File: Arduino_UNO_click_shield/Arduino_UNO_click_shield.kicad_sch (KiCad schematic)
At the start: 14 parts, among them J1 mikroBUS host connector, J2 mikroBUS host connector, J4 UPDI, U1 ATtiny1616-M

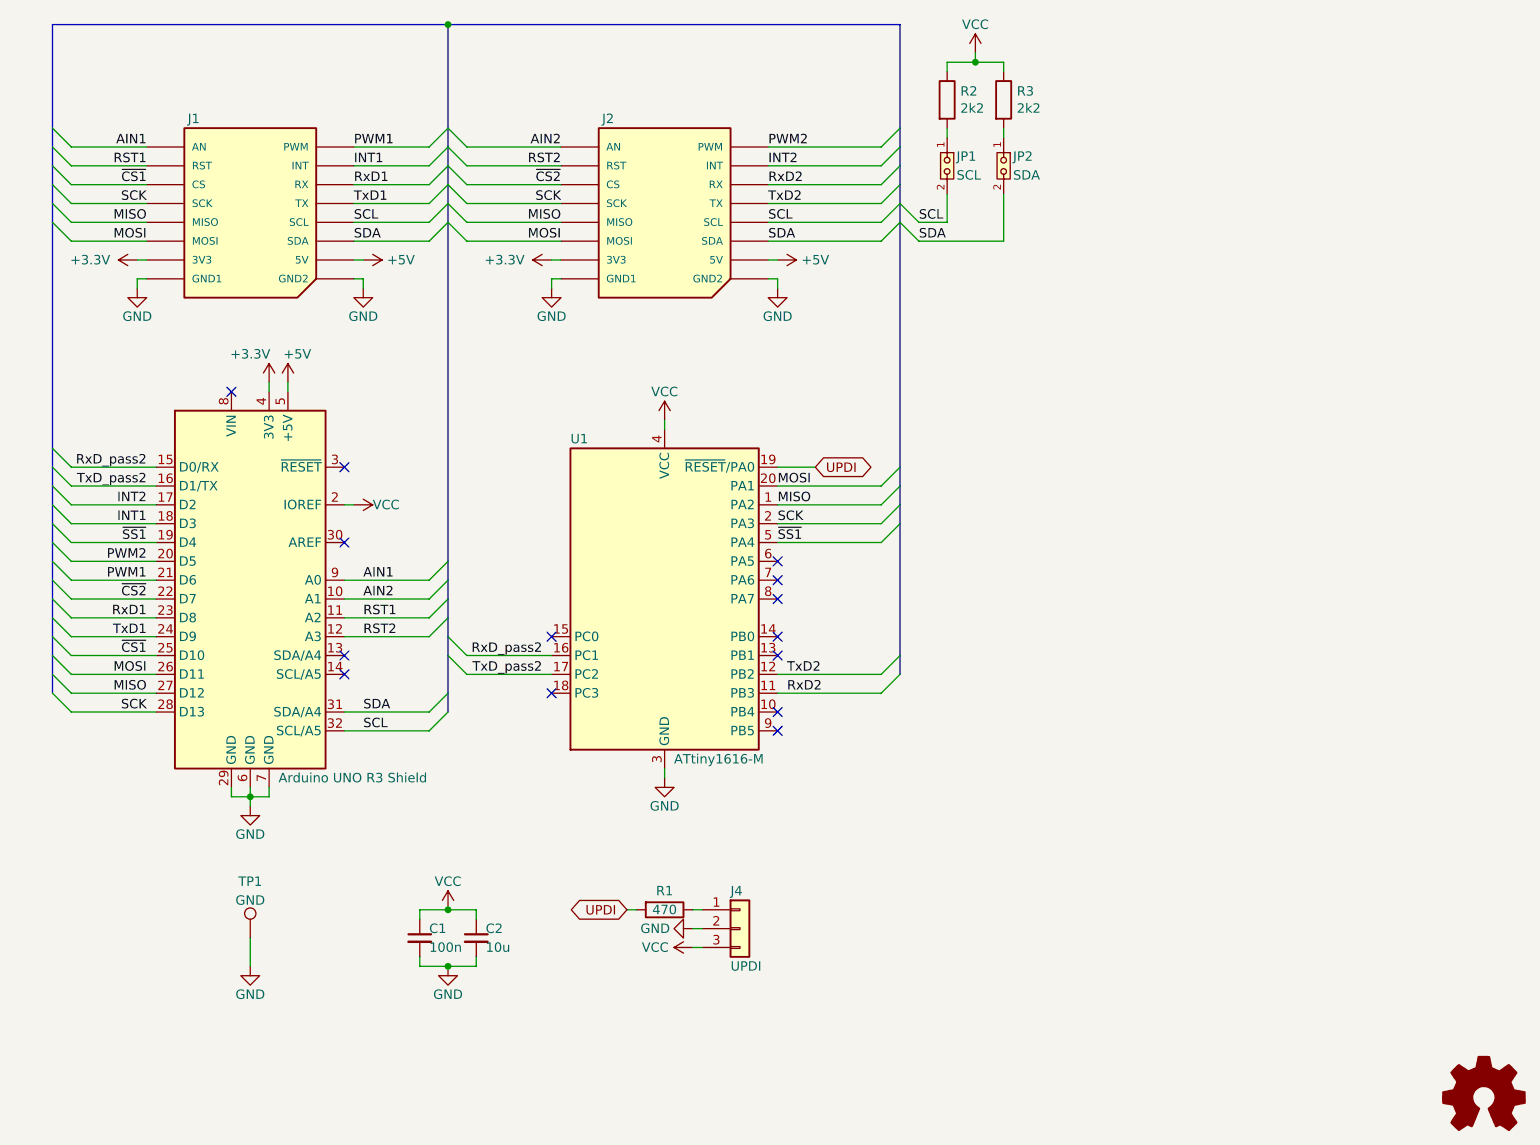
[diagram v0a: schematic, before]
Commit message: Arduino UNO Click shield v1.2
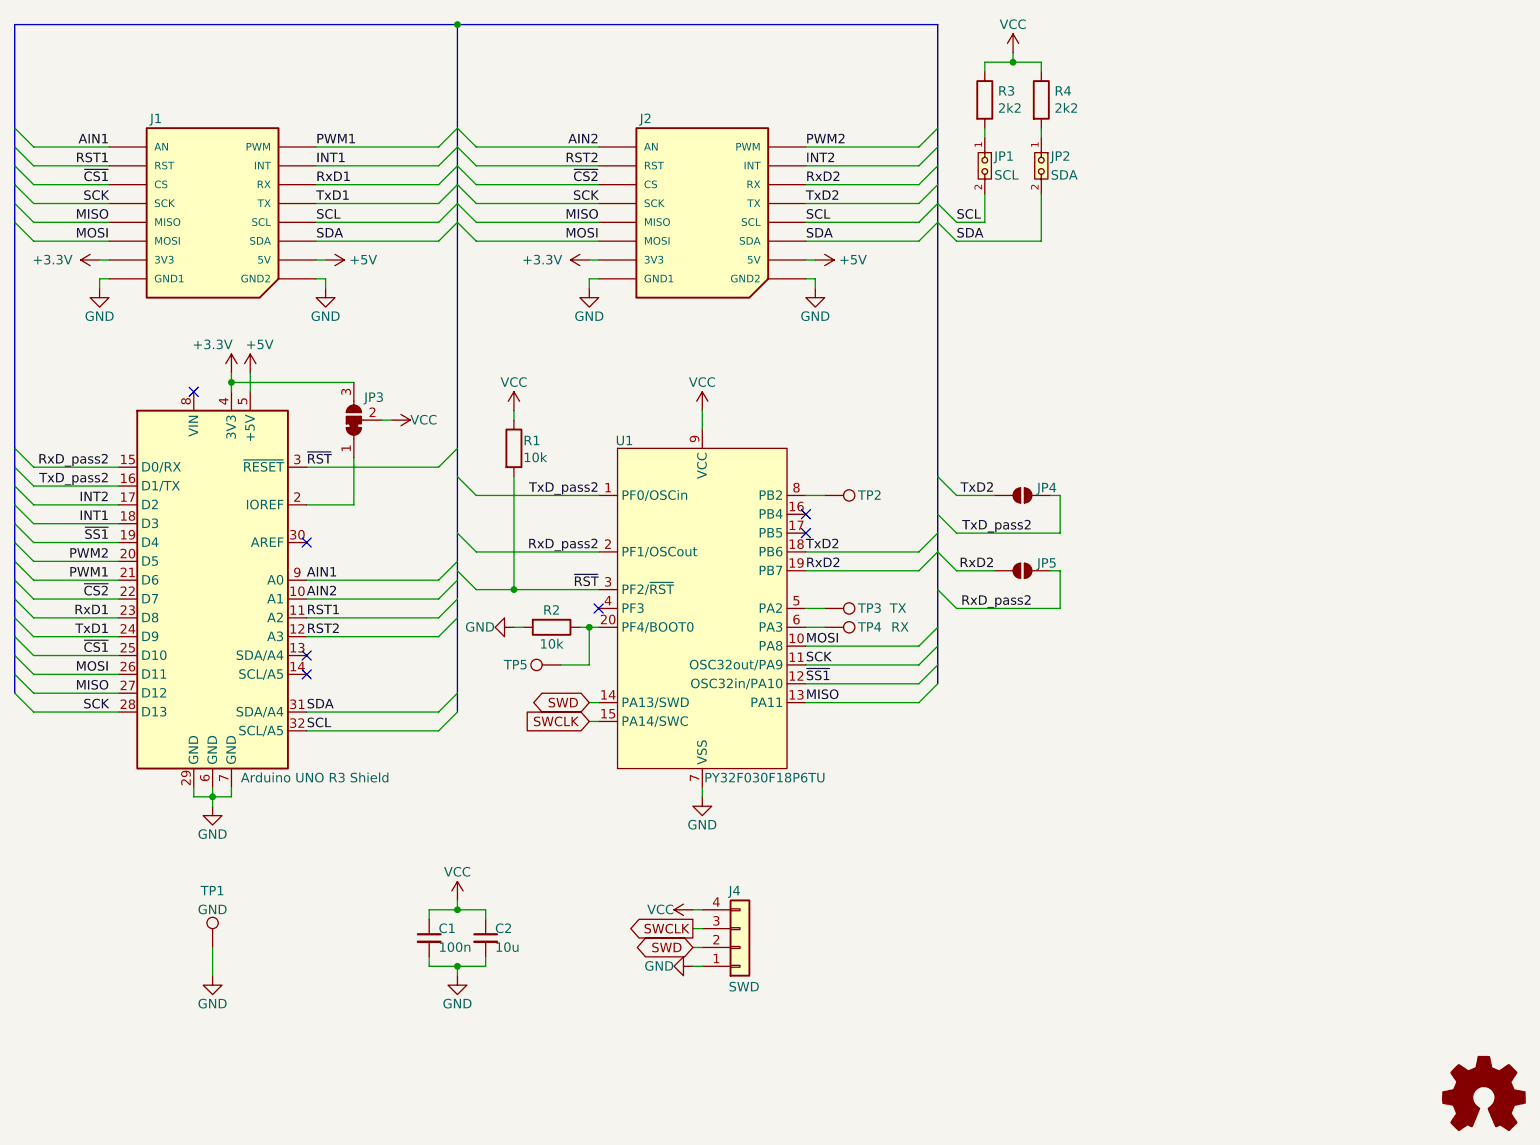
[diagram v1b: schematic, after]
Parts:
- removed J4: UPDI, footprints:PinHeader_1x03_P1.27mm_Vertical, symbol Connector_Generic:Conn_01x03
- removed U1: ATtiny1616-M, footprints:VQFN-20-1EP_3x3mm_P0.4mm_EP1.7x1.7mm, symbol MCU_Microchip_ATtiny:ATtiny1616-M
- added J4: SWD, footprints:PinHeader_1x04_P2.54mm_Horizontal, symbol Connector_Generic:Conn_01x04
- added JP3: VCC, footprints:SolderJumper-3_P1.3mm_Bridged12_RoundedPad1.0x1.5mm, symbol Jumper:SolderJumper_3_Bridged12
- added JP4: TX, footprints:SolderJumper-2_P1.3mm_Open_RoundedPad1.0x1.5mm, symbol Jumper:SolderJumper_2_Open
- added JP5: RX, footprints:SolderJumper-2_P1.3mm_Open_RoundedPad1.0x1.5mm, symbol Jumper:SolderJumper_2_Open
- added R1: 10k, footprints:R_0805_2012Metric, symbol archive:Device_R
- added TP2, TP5: ~, footprints:TestPoint_Pad_D1.0mm, symbol Connector:TestPoint
- added TP3: TX, footprints:TestPoint_Pad_D1.0mm, symbol Connector:TestPoint
- added TP4: RX, footprints:TestPoint_Pad_D1.0mm, symbol Connector:TestPoint
- added U1: PY32F030F18P6TU, Package_SO:TSSOP-20_4.4x6.5mm_P0.65mm, symbol various:PY32F030F1xP
- J1, J2: LCSC ----- -> C429957
- JP1, JP2: LCSC ----- -> C27985187
- R2: renamed from R1; value 470 -> 10k; LCSC C17710 -> C17414
- renumbered R2 to R3, R3 to R4
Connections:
- net UPDI is gone; now on net GND: R2.2
- net +3.3V: now also JP3.3 (B)
- net GND: now also J4.1 (Pin_1), U1.7 (VSS)
- net MISO: now also U1.13 (PA11)
- net MOSI: now also U1.10 (PA8)
- net RxD2: now also JP5.1 (A), U1.19 (PB7)
- net RxD_pass2: now also JP5.2 (B), U1.2 (PF1/OSCout)
- net SCK: now also U1.11 (OSC32out/PA9)
- net TxD2: now also JP4.1 (A), U1.18 (PB6)
- net TxD_pass2: now also JP4.2 (B), U1.1 (PF0/OSCin)
- net VCC: now also J4.4 (Pin_4), JP3.2 (C), R1.1, U1.9 (VCC); no longer A1.2 (IOREF)
- net ~{SS1}: now also U1.12 (OSC32in/PA10)
- net at R2.1: now also TP5.1, U1.20 (PF4/BOOT0)
- net ~{RST}: now reaches A1.3 (~{RESET})
- net ~{RST}: now also R1.2, U1.3 (PF2/~{RST})
- new net: TP4.1, U1.6 (PA3)
- new net: TP3.1, U1.5 (PA2)
- new net: TP2.1, U1.8 (PB2)
- new net: A1.2 (IOREF), JP3.1 (A)
- new net SWCLK: J4.3 (Pin_3), U1.15 (PA14/SWC)
- new net SWD: J4.2 (Pin_2), U1.14 (PA13/SWD)
- no-connect marks 14 -> 7
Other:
- company: © 2023 MPro -> © 2023-2025 MPro
- moved on the sheet: C1, C2, J1, J2, JP1, JP2, R2, R3, R4, TP1
